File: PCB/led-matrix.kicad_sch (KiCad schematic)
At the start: 21 parts, among them J1 Conn_02x03_Odd_Even

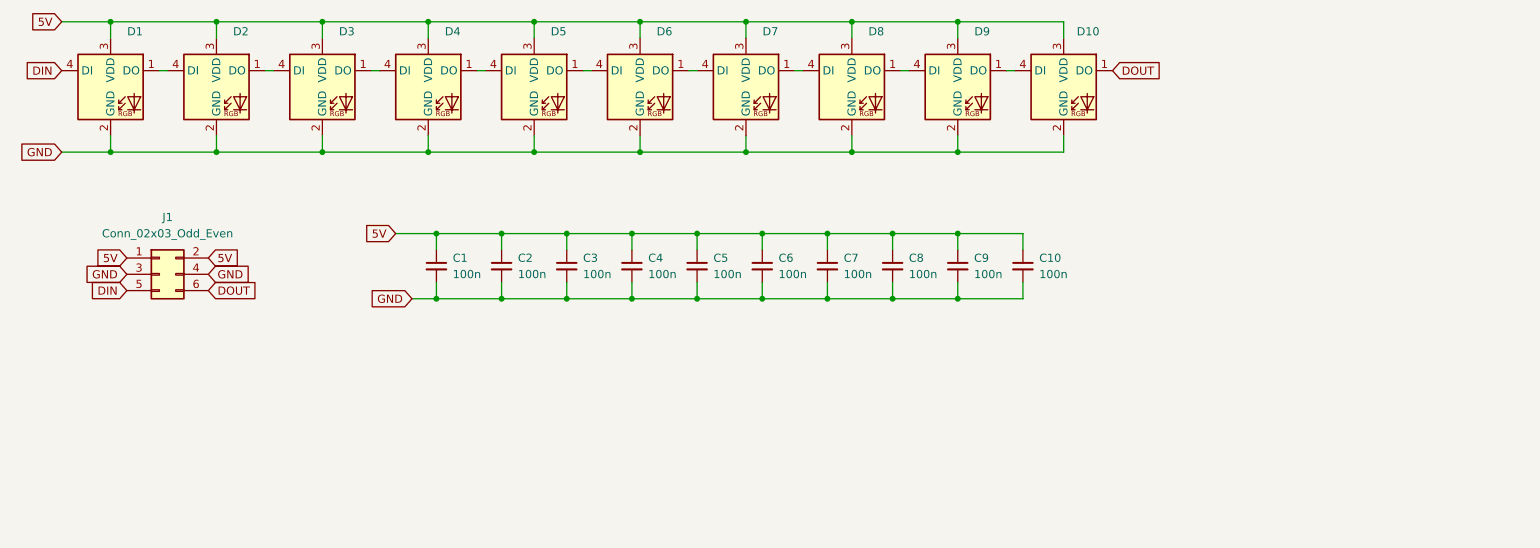
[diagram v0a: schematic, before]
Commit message: Layout board
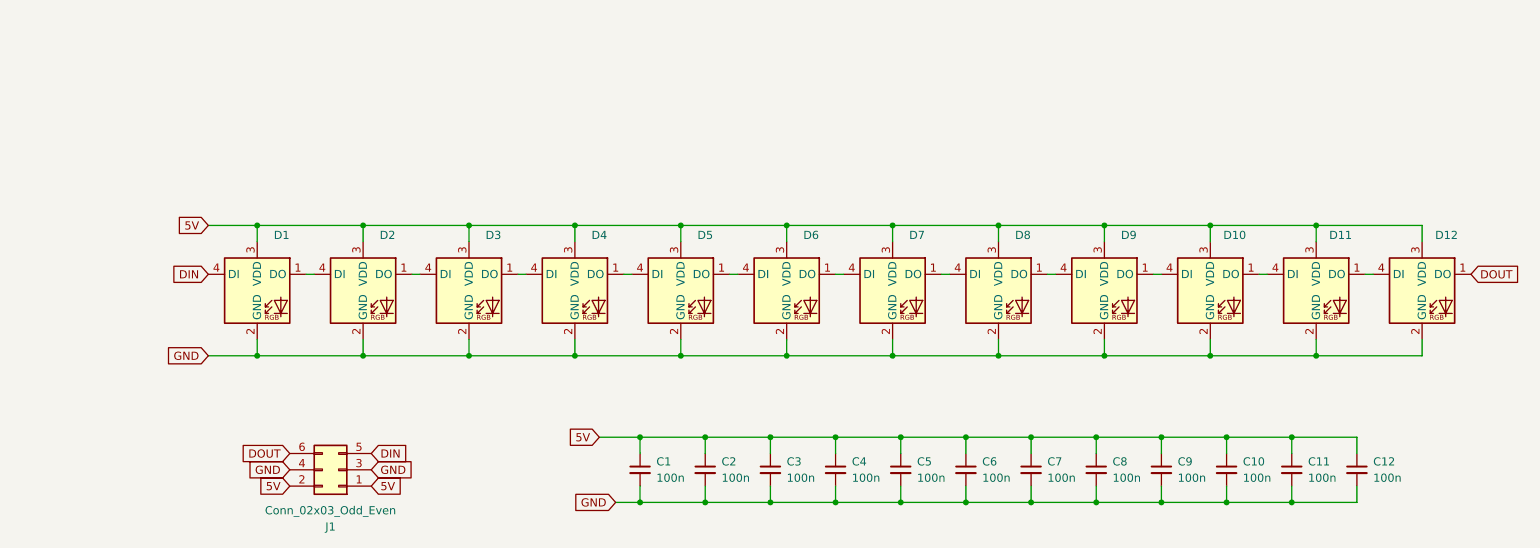
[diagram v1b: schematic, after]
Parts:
- added C11, C12: 100n, Capacitor_SMD:C_0603_1608Metric, symbol Device:C_Small
- added D11, D12: APA-106-F5, WS2812D:WS2812D, symbol LED:APA-106-F5
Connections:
- net 5V: now also C11.1, C12.1, D11.3 (VDD), D12.3 (VDD)
- net DOUT: now also D12.1 (DO); no longer D10.1 (DO)
- net GND: now also C11.2, C12.2, D11.2 (GND), D12.2 (GND)
- new net: D11.1 (DO), D12.4 (DI)
- new net: D10.1 (DO), D11.4 (DI)
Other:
- moved on the sheet: C1, C10, C2, C3, C4, C5, C6, C7, C8, C9, D1, D2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

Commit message: Resolve ground plane island issue
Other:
- title: (none) -> LED Matrix
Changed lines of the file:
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@@
 	(generator_version "8.0")
 	(paper "A4")
+	(title_block
+		(title "LED Matrix")
+		(date "2025-07-13")
+		(rev "0.2")
+	)
 	(junction
 		(at 215.9 111.76)
